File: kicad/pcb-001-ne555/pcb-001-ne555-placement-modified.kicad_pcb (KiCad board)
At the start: 2 copper layers, 14 parts, among them J1 +5 V / GND power input, U1 NE555D

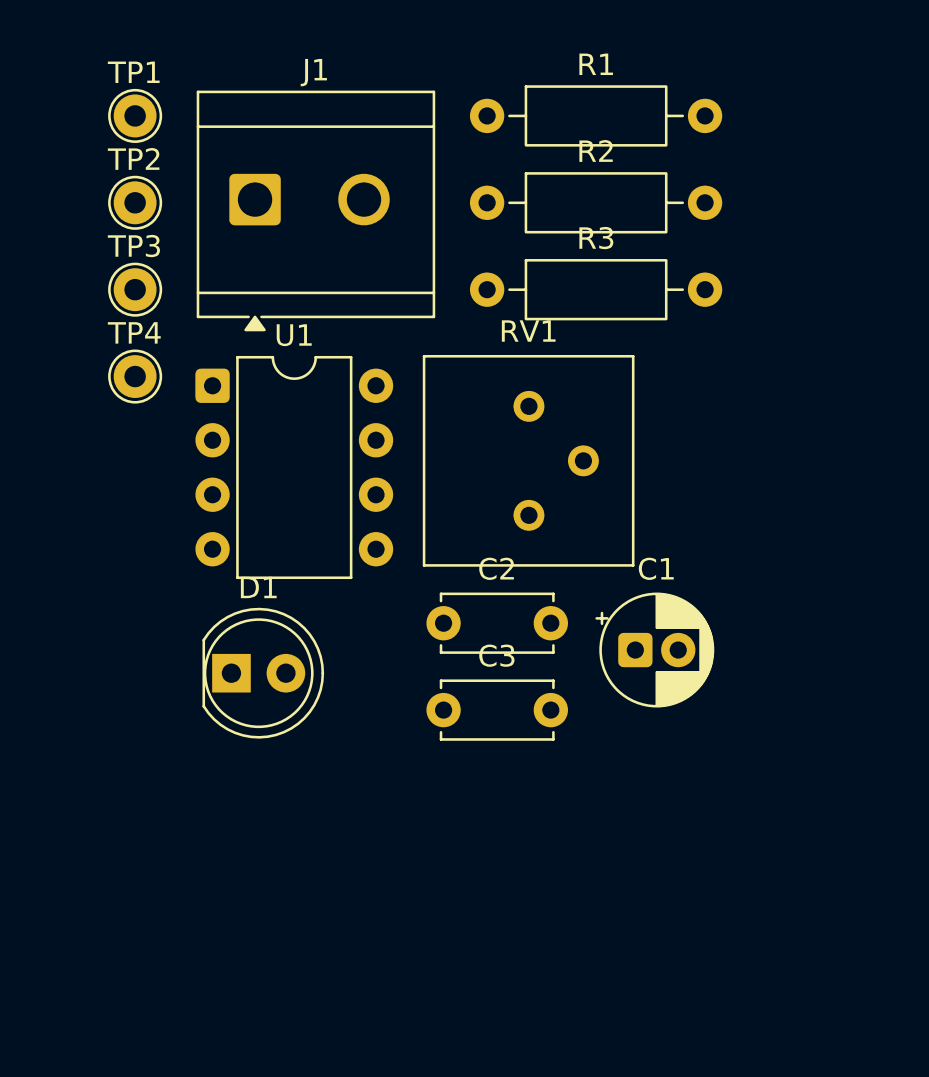
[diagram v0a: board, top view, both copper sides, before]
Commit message: Update project files 2026-08-16 01:39:38
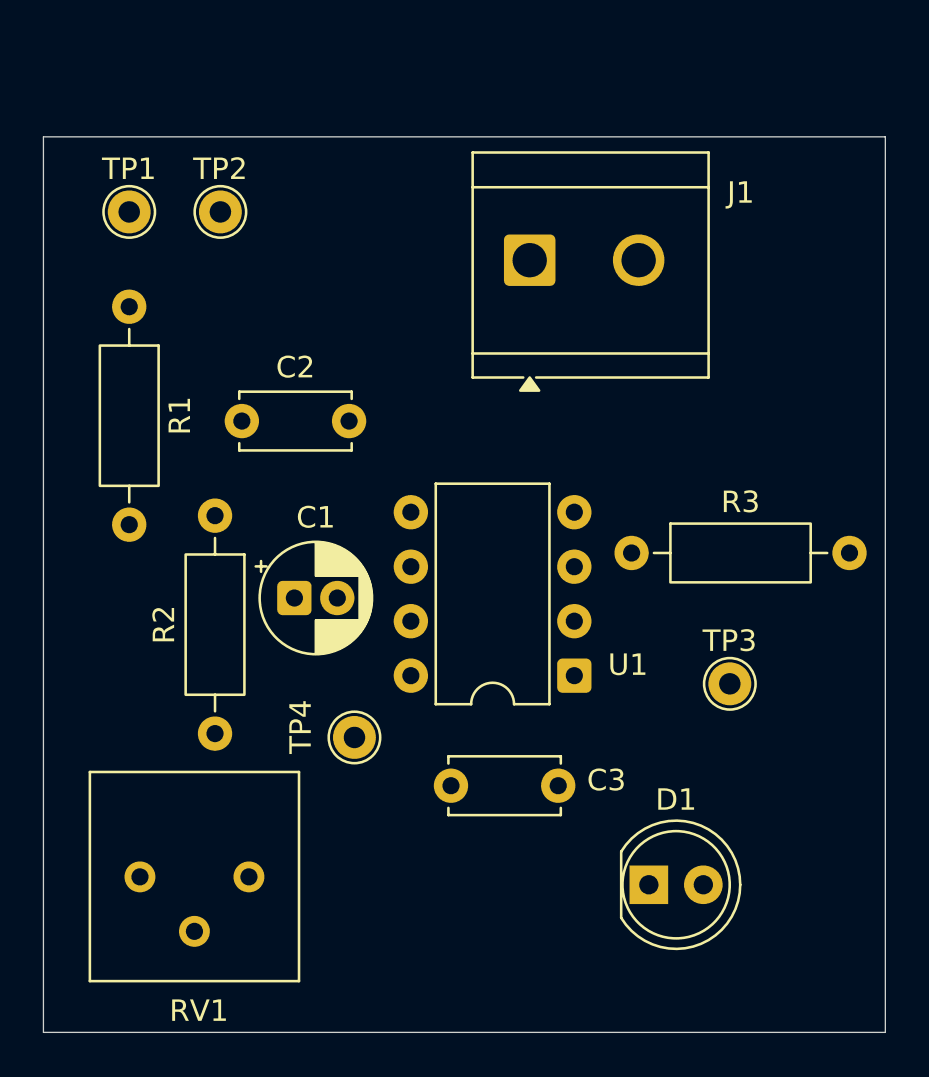
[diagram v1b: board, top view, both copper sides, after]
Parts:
- moved TP3 33.3 mm to (134.5, 108.0)
- moved RV1 24.8 mm to (107.0, 117.0), turned to -90 degrees
- moved D1 21.8 mm to (130.7, 117.4)
- moved U1 21.6 mm to (127.2, 107.6), turned to 180 degrees
- moved TP4 19.7 mm to (117.0, 110.5)
- moved R2 19.3 mm to (110.5, 100.2), turned to -90 degrees
- moved R1 18.9 mm to (106.5, 90.4), turned to -90 degrees
- moved C1 16.1 mm to (114.2, 104.0)
- moved R3 14.0 mm to (129.9, 101.9)
- moved C2 13.3 mm to (111.8, 95.8)
- moved J1 13.1 mm to (125.2, 88.2)
- moved TP1 4.48 mm to (106.5, 86.0)
- moved TP2 4.00 mm to (110.8, 86.0)
- moved C3 3.54 mm to (121.5, 112.8)
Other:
- board outline added: 39.2 x 41.8 mm
